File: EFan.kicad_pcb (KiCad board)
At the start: 2 copper layers, 48.9 x 38.1 mm, 46 parts, among them J1 Conn_01x04_Male, J2 Conn_01x03_Male, M1 Fan, Q1 TIP41, SW1 SW_Push, U1 STM32F030F4Px, U2 LM358, U3 MC34063AD

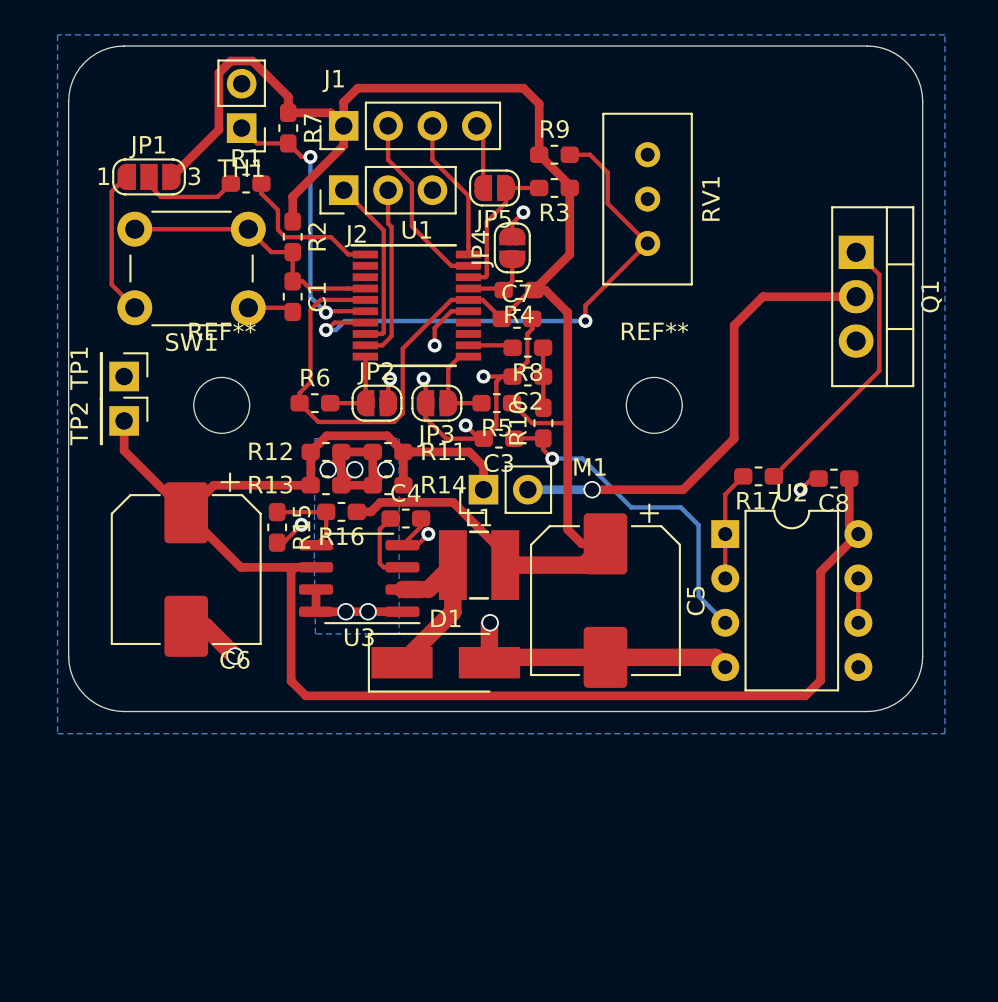
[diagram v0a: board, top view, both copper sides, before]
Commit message: production 2
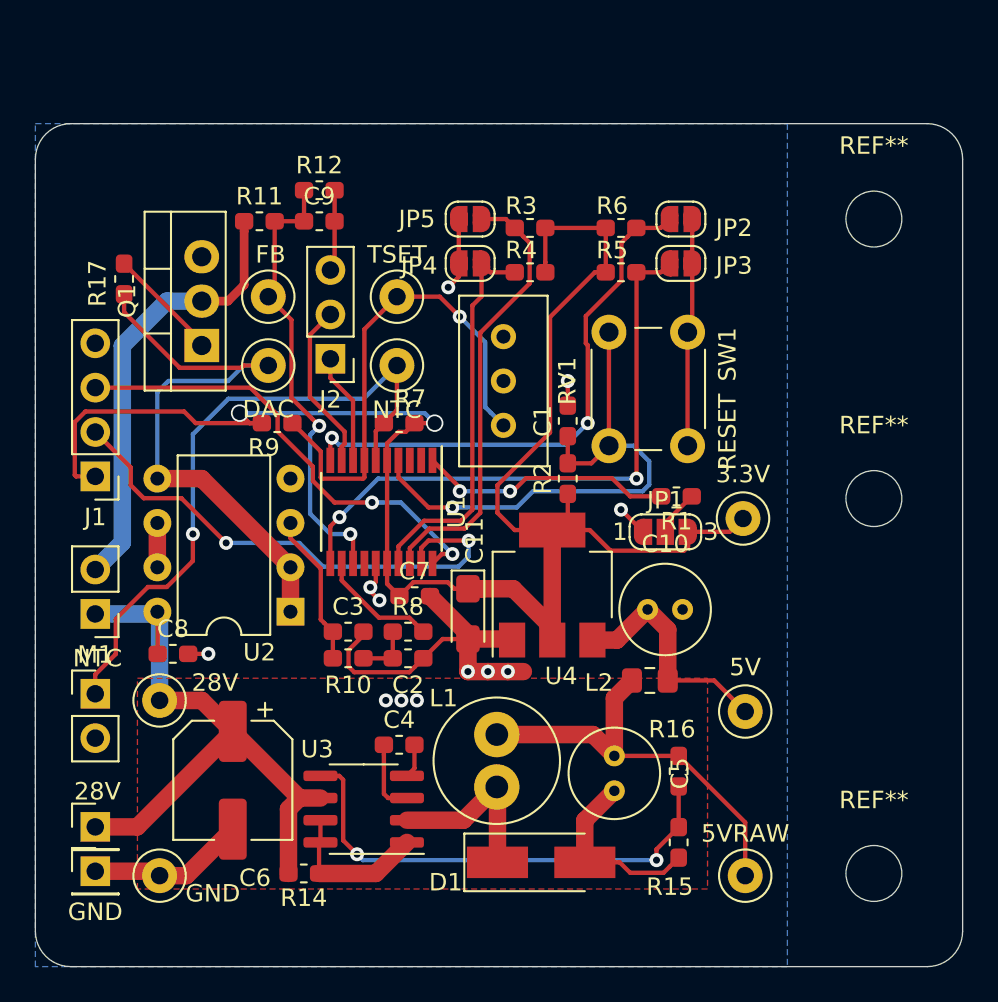
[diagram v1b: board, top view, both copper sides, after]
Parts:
- removed R13: 3R3, Resistor_SMD:R_0603_1608Metric_Pad1.05x0.95mm_HandSolder
- removed the REF** at (79.2, 102.5)
- removed the REF** at (104.0, 102.5)
- added C10: 100u, EFan:C_Radial_D5.0mm_H7.0mm_P2.00mm, F.Cu at (103.6, 114.2)
- added C11: 22u, EFan:CP_EIA-3216-18_Kemet-A_Pad1.58x1.35mm_HandSolder, F.Cu at (93.3, 114.4)
- added C9: 104, Capacitor_SMD:C_0603_1608Metric_Pad1.05x0.95mm_HandSolder, F.Cu at (84.8, 91.9)
- added L2: 1u, Inductor_SMD:L_0805_2012Metric_Pad1.15x1.40mm_HandSolder, F.Cu at (103.8, 118.2)
- added REF**: MountingHole_3.2mm_M3, MountingHole:MountingHole_3.2mm_M3, F.Cu at (116.6, 107.8)
- added REF**: MountingHole_3.2mm_M3, MountingHole:MountingHole_3.2mm_M3, F.Cu at (116.6, 129.3)
- added REF**: MountingHole_3.2mm_M3, MountingHole:MountingHole_3.2mm_M3, F.Cu at (116.6, 91.8)
- added TP10: 5V, TestPoint:TestPoint_Loop_D2.50mm_Drill1.0mm, F.Cu at (109.2, 120.0)
- added TP11: 3.3V, TestPoint:TestPoint_Loop_D2.50mm_Drill1.0mm, F.Cu at (109.1, 109.0)
- added TP3: GND, Connector_PinHeader_2.54mm:PinHeader_1x01_P2.54mm_Vertical, F.Cu at (72.0, 129.2)
- added TP4: DAC, TestPoint:TestPoint_Loop_D2.50mm_Drill1.0mm, F.Cu at (81.9, 100.2)
- added TP5: 28V, Connector_PinHeader_2.54mm:PinHeader_1x01_P2.54mm_Vertical, F.Cu at (72.0, 126.6)
- added TP6: FB, TestPoint:TestPoint_Loop_D2.50mm_Drill1.0mm, F.Cu at (81.9, 96.3)
- added TP7: 28V Loop, TestPoint:TestPoint_Loop_D2.50mm_Drill1.0mm, F.Cu at (75.7, 119.4)
- added TP8: GND Loop, TestPoint:TestPoint_Loop_D2.50mm_Drill1.0mm, F.Cu at (75.7, 129.4)
- added TP9: 5VRAW, TestPoint:TestPoint_Loop_D2.50mm_Drill1.0mm, F.Cu at (109.2, 129.4)
- added U4: AMS1117-3.3, Package_TO_SOT_SMD:SOT-223-3_TabPin2, F.Cu at (98.2, 112.8)
- C5: value 220u -> 100u; footprint Capacitor_SMD:CP_Elec_8x10 -> EFan:C_Radial_D5.0mm_H7.0mm_P2.00mm
- C6: value 100u -> 47u; footprint Capacitor_SMD:CP_Elec_8x10 -> EFan:CP_Elec_6.3x5.4
- D1: value SS34 -> SS24
- L1: value 220u -> 1m; footprint EFan:SMD,4.5x4x3.2mm Inductor -> EFan:L_Radial_D7.0mm_P3.00mm
- R11: value 3R3 -> 126k
- R12: value 3R3 -> 143
- R14: value 3R3 -> 2R7
- R15: value 6.8k -> 12k
- R16: value 11k -> 36k
- TH1: value Thermistor_NTC -> NTC
- TP1: value TestPoint -> NTC; footprint Connector_PinHeader_2.54mm:PinHeader_1x01_P2.54mm_Vertical -> TestPoint:TestPoint_Loop_D2.50mm_Drill1.0mm
- TP2: value TestPoint -> TSET; footprint Connector_PinHeader_2.54mm:PinHeader_1x01_P2.54mm_Vertical -> TestPoint:TestPoint_Loop_D2.50mm_Drill1.0mm
- moved C8 39.2 mm to (76.5, 116.7), turned to 0 degrees
- moved R17 38.0 mm to (73.7, 95.2), turned to 270 degrees
- moved Q1 37.8 mm to (78.1, 99.1), turned to 90 degrees
- moved JP1 35.9 mm to (104.6, 109.7)
- moved TH1 33.5 mm to (72.0, 119.0), turned to 0 degrees
- moved R1 30.5 mm to (105.3, 107.7), turned to 180 degrees
- moved R15 29.2 mm to (105.4, 127.5)
- moved U2 25.3 mm to (83.2, 114.3), turned to 180 degrees
- moved SW1 25.2 mm to (105.9, 98.3), turned to 270 degrees
- moved J1 24.6 mm to (72.0, 106.6), turned to 180 degrees
- moved R16 24.4 mm to (105.4, 123.4), turned to 270 degrees
- moved M1 23.3 mm to (72.0, 114.4), turned to 180 degrees
- moved R14 22.7 mm to (83.9, 129.3), turned to 0 degrees
- moved R9 22.1 mm to (82.4, 103.5)
- moved R2 21.0 mm to (99.1, 106.7), turned to 90 degrees
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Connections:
- C5 pad 1: VCC -> Net-(C5-Pad1)
- L1 pad 2: VCC -> Net-(C5-Pad1)
- R11 pad 1: +28V -> Net-(M1-Pad2)
- R11 pad 2: Net-(R11-Pad2) -> Net-(C9-Pad1)
- R12 pad 1: +28V -> Net-(C9-Pad1)
- R12 pad 2: Net-(R11-Pad2) -> GND
- R14 pad 2: Net-(R11-Pad2) -> /Step Down Power/Sensed28
- R16 pad 1: VCC -> Net-(C5-Pad1)
- R17 pad 2: Net-(R17-Pad2) -> /DAC
- TP1 pad 1: GND -> Net-(R7-Pad2)
- TP2 pad 1: +28V -> Net-(R9-Pad2)
- U1 pad 13: Net-(U1-Pad13) -> Net-(C9-Pad1)
- U2 pad 1: Net-(R17-Pad2) -> /DAC
- U2 pad 2: Net-(R17-Pad2) -> /DAC
- U2 pad 5: GND -> /DAC
- U3 pad 1: Net-(R11-Pad2) -> /Step Down Power/Sensed28
- U3 pad 7: Net-(R11-Pad2) -> /Step Down Power/Sensed28
- U3 pad 8: Net-(R11-Pad2) -> /Step Down Power/Sensed28
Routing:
- net +28V: track 91.6 -> 37.4 mm
- net /DAC: track 0.00 -> 34.9 mm
- net /DIP2: track 5.34 -> 34.7 mm, vias 0 -> 2
- net /DIP1: track 4.70 -> 31.2 mm, vias 0 -> 2
- net Net-(C9-Pad1): track 0.00 -> 26.3 mm, vias 0 -> 2
- net Net-(C5-Pad1): track 0.00 -> 24.1 mm
- net Net-(R15-Pad1): track 4.96 -> 28.0 mm, vias 0 -> 2
- net Net-(R7-Pad2): track 16.2 -> 37.1 mm, vias 2 -> 1
- net /SWDIO: track 10.5 -> 30.1 mm, vias 0 -> 2
- net /SWCLK: track 8.22 -> 26.8 mm, vias 0 -> 2
- net /DIP3: track 4.02 -> 22.5 mm
- net Net-(R11-Pad2): track 17.4 -> 0.00 mm, vias 5 -> 0
- net /DIP4: track 8.47 -> 25.7 mm
- net Net-(C1-Pad1): track 15.6 -> 31.4 mm, vias 0 -> 1
- net VCC: track 115.7 -> 101.7 mm, vias 0 -> 2
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- added copper zone on F.Cu, net GND
- removed copper zone on B.Cu, net Net-(R11-Pad2)
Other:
- board size 48.9 x 38.1 mm -> 53.1 x 48.3 mm
